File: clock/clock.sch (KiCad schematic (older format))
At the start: 13 parts, among them J1 SWD, U1 iv12, U2 iv12, U3 iv12, U4 iv12, U5 STM32F103C8Tx, Y1 8Mhz, Y2 32.768khz

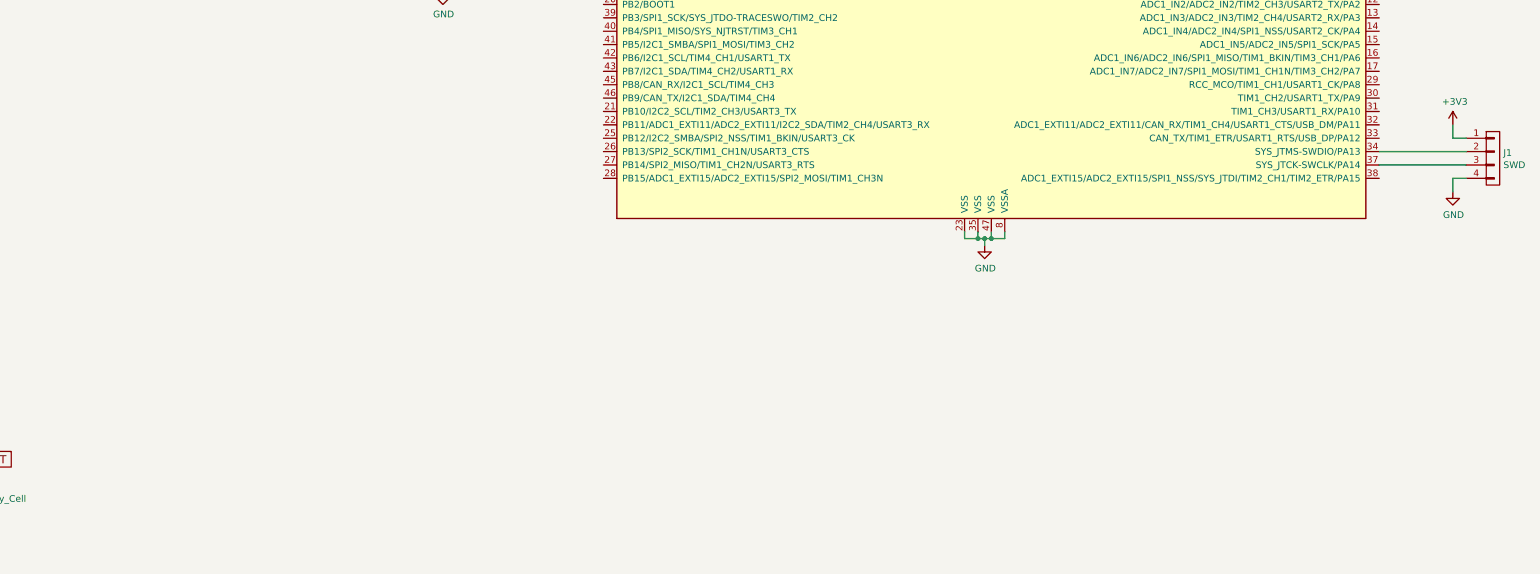
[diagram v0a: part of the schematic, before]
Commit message: Start of power design
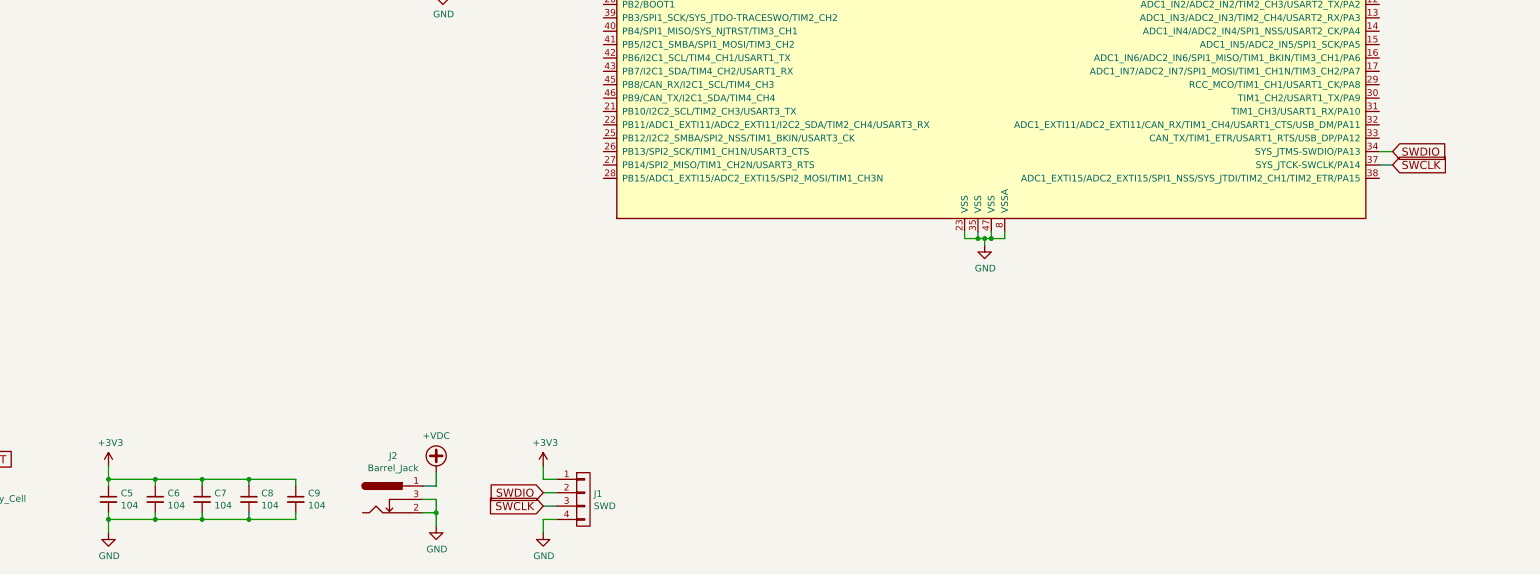
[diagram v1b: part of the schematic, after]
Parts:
- added C5, C6, C7, C8, C9: 104, Capacitors_SMD:C_0603_HandSoldering, symbol C_Small
- added J2: Barrel_Jack, Connectors:Barrel_Jack_CUI_PJ-036AH-SMT, symbol Barrel_Jack
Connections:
- net +3V3: now also C5.1, C6.1, C7.1, C8.1, C9.1
- net GND: now also C5.2, C6.2, C7.2, C8.2, C9.2, J2.2, J2.3
- net SWDIO: now reaches J1.2 (P2), U5.34 (SYS_JTMS-SWDIO/PA13)
- net SWCLK: now reaches J1.3 (P3), U5.37 (SYS_JTCK-SWCLK/PA14)
- new net +VDC: J2.1
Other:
- moved on the sheet: J1
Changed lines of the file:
@@
 L CONN_01X04 J1
 U 1 1 5A920C48
-P 12350 8100
-F 0 "J1" H 12428 8141 50  0000 L CNN
-F 1 "SWD" H 12428 8050 50  0000 L CNN
-F 2 "Pin_Headers:Pin_Header_Straight_1x04_Pitch2.54mm" H 12350 8100 50  0001 C CNN
-F 3 "" H 12350 8100 50  0001 C CNN
-	1    12350 8100
-	1    0    0    -1
-$EndComp
-Wire Wire Line
-	11500 8050 12150 8050
-Wire Wire Line
-	11500 8150 12150 8150
+P 5550 10650
+F 0 "J1" H 5628 10691 50  0000 L CNN
+F 1 "SWD" H 5628 10600 50  0000 L CNN
+F 2 "Pin_Headers:Pin_Header_Straight_1x04_Pitch2.54mm" H 5550 10650 50  0001 C CNN
+F 3 "" H 5550 10650 50  0001 C CNN
+	1    5550 10650
+	1    0    0    -1
+$EndComp
 $Comp
 L GND #PWR013
 U 1 1 5A920F1C
-P 12050 8350
-F 0 "#PWR013" H 12050 8100 50  0001 C CNN
-F 1 "GND" H 12055 8177 50  0000 C CNN
-F 2 "" H 12050 8350 50  0001 C CNN
-F 3 "" H 12050 8350 50  0001 C CNN
-	1    12050 8350
-	1    0    0    -1
-$EndComp
-Wire Wire Line
-	12050 8350 12050 8250
-Wire Wire Line
-	12050 8250 12150 8250
+P 5250 10900
+F 0 "#PWR013" H 5250 10650 50  0001 C CNN
+F 1 "GND" H 5255 10727 50  0000 C CNN
+F 2 "" H 5250 10900 50  0001 C CNN
+F 3 "" H 5250 10900 50  0001 C CNN
+	1    5250 10900
+	1    0    0    -1
+$EndComp
+Wire Wire Line
+	5250 10900 5250 10800
+Wire Wire Line
+	5250 10800 5350 10800
 $Comp
 L +3V3 #PWR014
 U 1 1 5A920FA9
-P 12050 7850
-F 0 "#PWR014" H 12050 7700 50  0001 C CNN
-F 1 "+3V3" H 12065 8023 50  0000 C CNN
-F 2 "" H 12050 7850 50  0001 C CNN
-F 3 "" H 12050 7850 50  0001 C CNN
-	1    12050 7850
-	1    0    0    -1
-$EndComp
-Wire Wire Line
-	12050 7850 12050 7950
-Wire Wire Line
-	12050 7950 12150 7950
+P 5250 10400
+F 0 "#PWR014" H 5250 10250 50  0001 C CNN
+F 1 "+3V3" H 5265 10573 50  0000 C CNN
+F 2 "" H 5250 10400 50  0001 C CNN
+F 3 "" H 5250 10400 50  0001 C CNN
+	1    5250 10400
+	1    0    0    -1
+$EndComp
+Wire Wire Line
+	5250 10400 5250 10500
+Wire Wire Line
+	5250 10500 5350 10500
 Wire Wire Line
 	9500 2850 9500 2950
@@
 Wire Wire Line
 	850  10350 950  10350
+$Comp
+L C_Small C7
+U 1 1 5A92C1A1
+P 2700 10650
+F 0 "C7" H 2792 10696 50  0000 L CNN
+F 1 "104" H 2792 10605 50  0000 L CNN
+F 2 "Capacitors_SMD:C_0603_HandSoldering" H 2700 10650 50  0001 C CNN
+F 3 "" H 2700 10650 50  0001 C CNN
+	1    2700 10650
+	1    0    0    -1
+$EndComp
+$Comp
+L C_Small C8
+U 1 1 5A92C295
+P 3050 10650
+F 0 "C8" H 3142 10696 50  0000 L CNN
+F 1 "104" H 3142 10605 50  0000 L CNN
+F 2 "Capacitors_SMD:C_0603_HandSoldering" H 3050 10650 50  0001 C CNN
+F 3 "" H 3050 10650 50  0001 C CNN
+	1    3050 10650
+	1    0    0    -1
+$EndComp
+$Comp
+L C_Small C5
+U 1 1 5A92C32D
+P 2000 10650
+F 0 "C5" H 2092 10696 50  0000 L CNN
+F 1 "104" H 2092 10605 50  0000 L CNN
+F 2 "Capacitors_SMD:C_0603_HandSoldering" H 2000 10650 50  0001 C CNN
+F 3 "" H 2000 10650 50  0001 C CNN
+	1    2000 10650
+	1    0    0    -1
+$EndComp
+$Comp
+L C_Small C6
+U 1 1 5A92C333
+P 2350 10650
+F 0 "C6" H 2442 10696 50  0000 L CNN
+F 1 "104" H 2442 10605 50  0000 L CNN
+F 2 "Capacitors_SMD:C_0603_HandSoldering" H 2350 10650 50  0001 C CNN
+F 3 "" H 2350 10650 50  0001 C CNN
+	1    2350 10650
+	1    0    0    -1
+$EndComp
+Wire Wire Line
+	2000 10400 2000 10550
+Wire Wire Line
+	2000 10500 3400 10500
+Wire Wire Line
+	2350 10500 2350 10550
+Wire Wire Line
+	2700 10500 2700 10550
+Connection ~ 2350 10500
+Wire Wire Line
+	3050 10500 3050 10550
+Connection ~ 2700 10500
+Wire Wire Line
+	2000 10750 2000 10900
+Wire Wire Line
+	2000 10800 3400 10800
+Wire Wire Line
+	2350 10800 2350 10750
+Wire Wire Line
+	2700 10800 2700 10750
+Connection ~ 2350 10800
+Wire Wire Line
+	3050 10800 3050 10750
+Connection ~ 2700 10800
+$Comp
+L GND #PWR019
+U 1 1 5A92C5A3
+P 2000 10900
+F 0 "#PWR019" H 2000 10650 50  0001 C CNN
+F 1 "GND" H 2005 10727 50  0000 C CNN
+F 2 "" H 2000 10900 50  0001 C CNN
+F 3 "" H 2000 10900 50  0001 C CNN
+	1    2000 10900
+	1    0    0    -1
+$EndComp
+$Comp
+L +3V3 #PWR020
+U 1 1 5A92C6B7
+P 2000 10400
+F 0 "#PWR020" H 2000 10250 50  0001 C CNN
+F 1 "+3V3" H 2015 10573 50  0000 C CNN
+F 2 "" H 2000 10400 50  0001 C CNN
+F 3 "" H 2000 10400 50  0001 C CNN
+	1    2000 10400
+	1    0    0    -1
+$EndComp
+Connection ~ 2000 10500
+Connection ~ 2000 10800
+$Comp
+L C_Small C9
+U 1 1 5A92CBFF
+P 3400 10650
+F 0 "C9" H 3492 10696 50  0000 L CNN
+F 1 "104" H 3492 10605 50  0000 L CNN
+F 2 "Capacitors_SMD:C_0603_HandSoldering" H 3400 10650 50  0001 C CNN
+F 3 "" H 3400 10650 50  0001 C CNN
+	1    3400 10650
+	1    0    0    -1
+$EndComp
+Wire Wire Line
+	3400 10500 3400 10550
+Connection ~ 3050 10500
+Wire Wire Line
+	3400 10800 3400 10750
+Connection ~ 3050 10800
+$Comp
+L Barrel_Jack J2
+U 1 1 5A92CF0D
+P 4050 10650
+F 0 "J2" H 4128 10975 50  0000 C CNN
+F 1 "Barrel_Jack" H 4128 10884 50  0000 C CNN
+F 2 "Connectors:Barrel_Jack_CUI_PJ-036AH-SMT" H 4100 10610 50  0001 C CNN
+F 3 "~" H 4100 10610 50  0001 C CNN
+	1    4050 10650
+	1    0    0    -1
+$EndComp
+$Comp
+L GND #PWR021
+U 1 1 5A92CFDF
+P 4450 10850
+F 0 "#PWR021" H 4450 10600 50  0001 C CNN
+F 1 "GND" H 4455 10677 50  0000 C CNN
+F 2 "" H 4450 10850 50  0001 C CNN
+F 3 "" H 4450 10850 50  0001 C CNN
+	1    4450 10850
+	1    0    0    -1
+$EndComp
+Wire Wire Line
+	4350 10650 4450 10650
+Wire Wire Line
+	4450 10650 4450 10850
+Wire Wire Line
+	4350 10750 4450 10750
+Connection ~ 4450 10750
+$Comp
+L +VDC #PWR022
+U 1 1 5A92D129
+P 4450 10450
+F 0 "#PWR022" H 4450 10350 50  0001 C CNN
+F 1 "+VDC" H 4450 10725 50  0000 C CNN
+F 2 "" H 4450 10450 50  0001 C CNN
+F 3 "" H 4450 10450 50  0001 C CNN
+	1    4450 10450
+	1    0    0    -1
+$EndComp
+Wire Wire Line
+	4450 10450 4450 10550
+Wire Wire Line
+	4450 10550 4350 10550
+Text GLabel 11600 8050 2    60   Input ~ 0
+SWDIO
+Text GLabel 11600 8150 2    60   Input ~ 0
+SWCLK
+Text GLabel 5250 10600 0    60   Input ~ 0
+SWDIO
+Text GLabel 5250 10700 0    60   Input ~ 0
+SWCLK
+Wire Wire Line
+	5250 10600 5350 10600
+Wire Wire Line
+	5350 10700 5250 10700
+Wire Wire Line
+	11600 8050 11500 8050
+Wire Wire Line
+	11500 8150 11600 8150
 $EndSCHEMATC

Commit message: Moved around power features
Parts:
- removed J1: SWD, Pin_Headers:Pin_Header_Straight_1x04_Pitch2.54mm, symbol CONN_01X04
- removed J2: Barrel_Jack, Connectors:Barrel_Jack_CUI_PJ-036AH-SMT, symbol Barrel_Jack
- added J1: USB_OTG, Connectors_USB:USB_Micro-B_Molex_47346-0001, symbol clock-rescue:USB_OTG-conn1
- added R1, R2: 22R, Resistors_SMD:R_0603_HandSoldering, symbol clock-rescue:R_Small-device1
- added R3: 10k, Resistors_SMD:R_0603_HandSoldering, symbol clock-rescue:R_Small-device1
- BT1: symbol Battery_Cell -> clock-rescue:Battery_Cell-device1
- C1, C2, C3, C4, C5, C6, C7, C8, C9: symbol C_Small -> clock-rescue:C_Small-device1
- U1, U2, U3, U4: symbol iv12 -> clock-rescue:iv12-iv12
- U5: symbol STM32F103C8Tx -> clock-rescue:STM32F103C8Tx-MCU_ST_STM32
- Y1, Y2: symbol Crystal -> clock-rescue:Crystal-device1
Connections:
- net GND: now also J1.4 (ID), J1.5 (GND), J1.6 (Shield)
- net D-: now reaches U5.32 (ADC1_EXTI11/ADC2_EXTI11/CAN_RX/TIM1_CH4/USART1_CTS/USB_DM/PA11)
- net D-: now also R2.2
- net D+: now reaches U5.33 (CAN_TX/TIM1_ETR/USART1_RTS/USB_DP/PA12)
- net D+: now also R1.2, R3.2
- net SWCLK: no longer names the net of U5.37 (SYS_JTCK-SWCLK/PA14)
- net SWDIO: no longer names the net of U5.34 (SYS_JTMS-SWDIO/PA13)
- new net: J1.2 (D-), R2.1
- new net: J1.3 (D+), R1.1
- new net +5V: J1.1 (VBUS), R3.1
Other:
- moved on the sheet: C5, C6, C7, C8, C9
